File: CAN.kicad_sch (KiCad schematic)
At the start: 12 parts, among them U4 SIT65HVD230DR

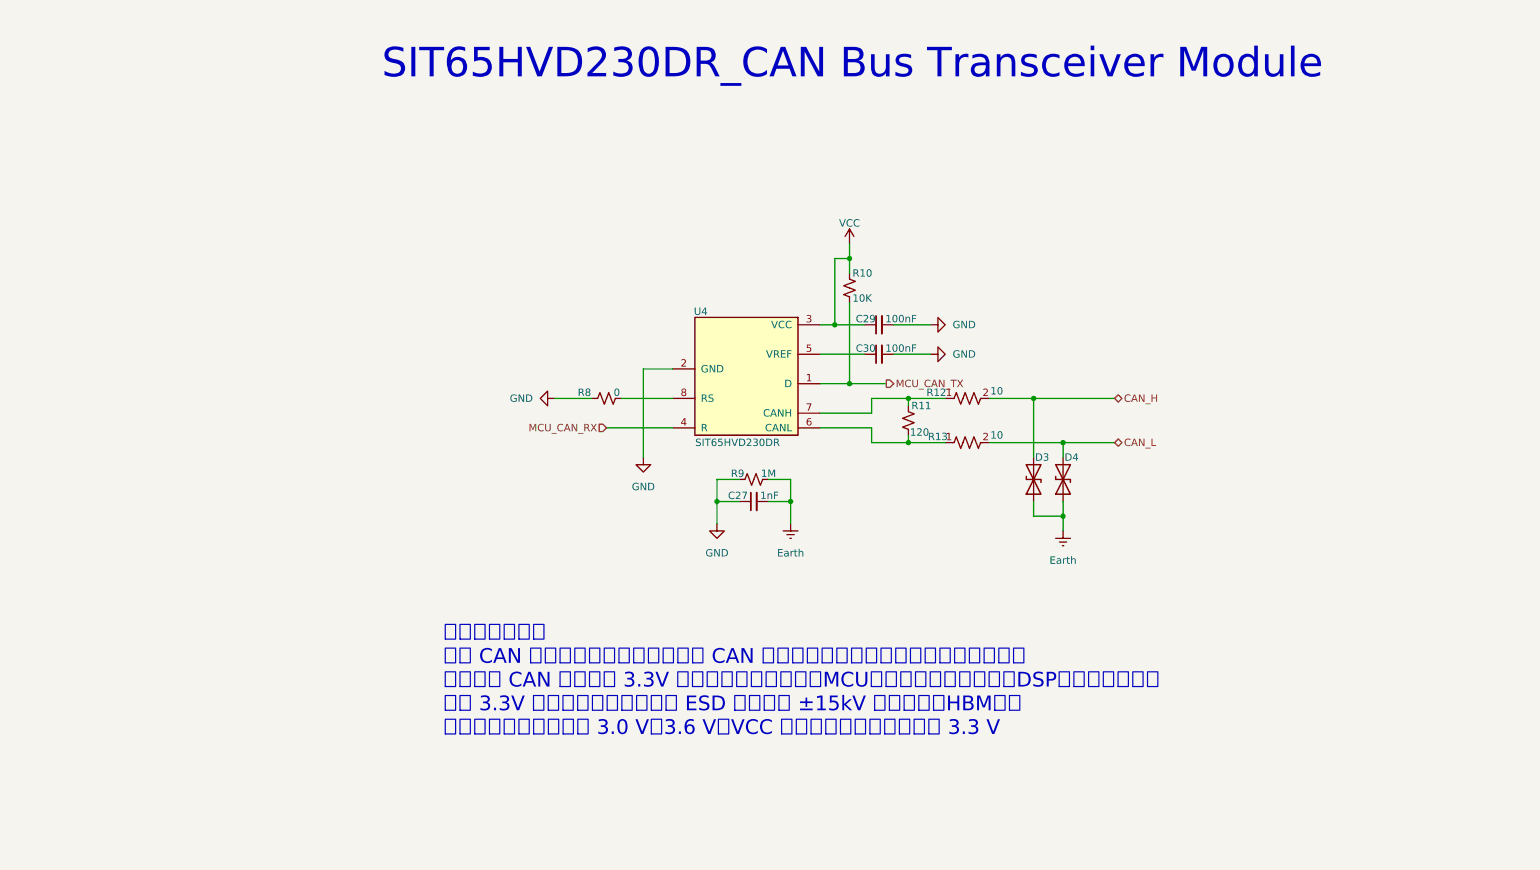
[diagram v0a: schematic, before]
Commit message: 更新原理图
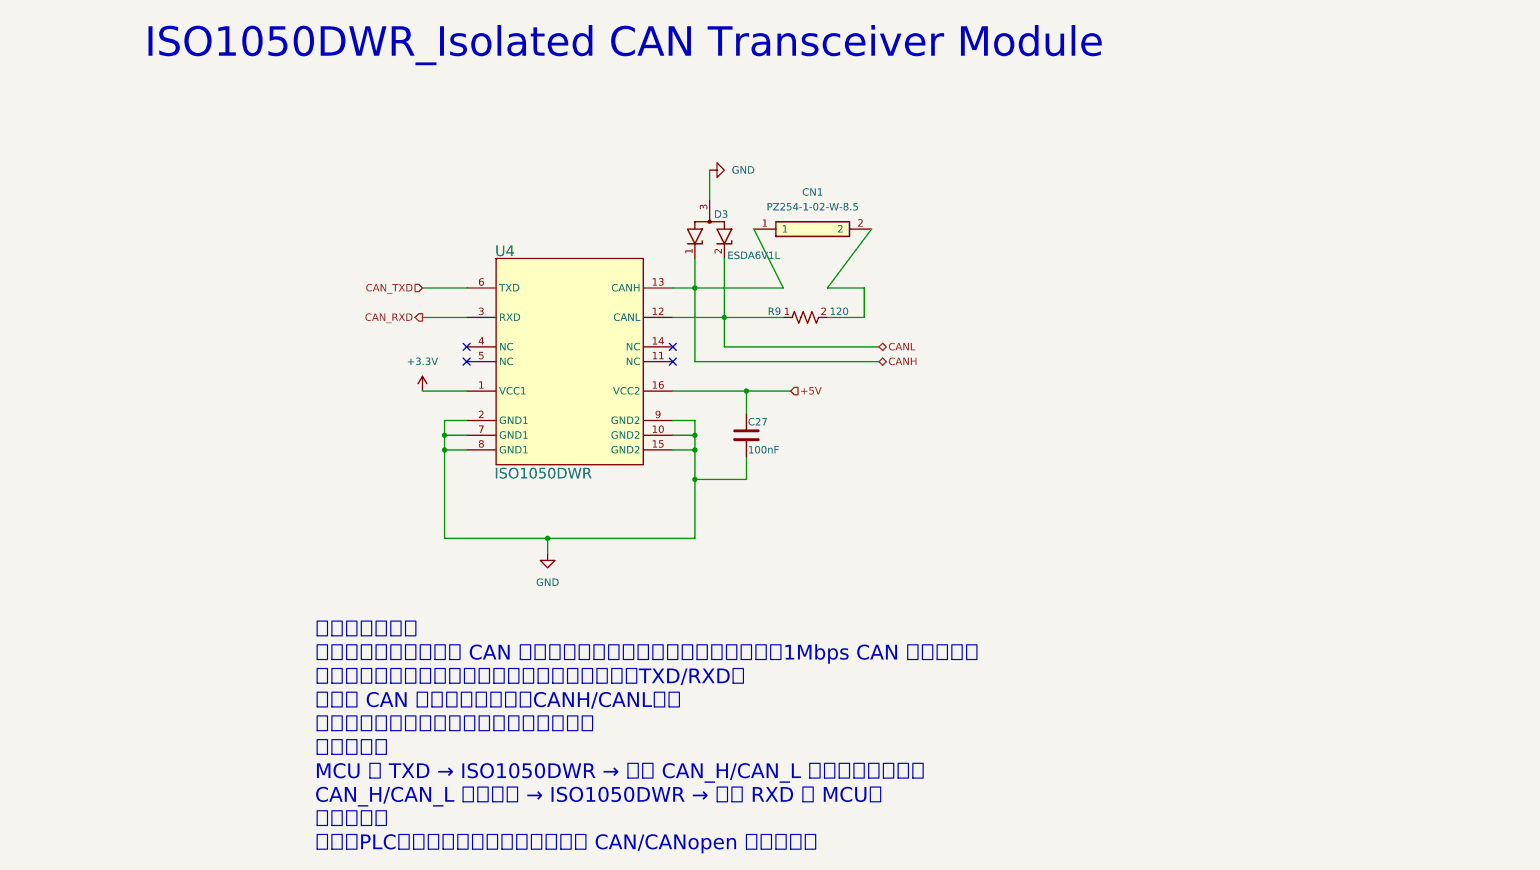
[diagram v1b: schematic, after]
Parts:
- removed C27: 1nF, kicad_community_lib:CC1206JKX7RDBB102, symbol CC1206JKX7RDBB102:CC1206JKX7RDBB102
- removed C29, C30: 100nF, kicad_api_lib:0402B104J160CT, symbol 0402B104J160CT:0402B104J160CT
- removed D3, D4: PESD12VV1BL-N, kicad_api_lib:PESD12VV1BL-N, symbol PESD12VV1BL-N:PESD12VV1BL-N
- removed R10: 10K, kicad_api_lib:AC0603JR-0710KL, symbol AC0603JR-0710KL:AC0603JR-0710KL
- removed R11: 120, kicad_api_lib:CRCW0603120RFKEA, symbol CRCW0603120RFKEA:CRCW0603120RFKEA
- removed R12, R13: 10, kicad_api_lib:AC0402FR-0710RL, symbol AC0402FR-0710RL:AC0402FR-0710RL
- removed R8: 0, kicad_api_lib:AC0603FR-070RL, symbol AC0603FR-070RL:AC0603FR-070RL
- removed R9: 1M, kicad_community_lib:RK73B1JTTD105J, symbol RK73B1JTTD105J:RK73B1JTTD105J
- removed U4: SIT65HVD230DR, kicad_api_lib:SIT65HVD230DR, symbol SIT65HVD230DR:SIT65HVD230DR
- added C27: 100nF, kicad_api_lib:CL05B104KB54PNC, symbol CL05B104KB54PNC:CL05B104KB54PNC
- added CN1: PZ254-1-02-W-8.5, kicad_api_lib:PZ254-1-02-W-8.5, symbol PZ254-1-02-W-8.5:FWF12507-S02B24W5B
- added D3: ESDA6V1L, kicad_api_lib:ESDA6V1L, symbol ESDA6V1L:ESDA6V1L
- added R9: 120, kicad_api_lib:0603WAF1200T5E, symbol 0603WAF1200T5E:0603WAF1200T5E
- added U4: ISO1050DWR, kicad_api_lib:ISO1050DWR, symbol ISO1050DWR:ISO1050DWR
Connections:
- net GND: now also C27.2, D3.3 (A), U4.10 (GND2), U4.15 (GND2), U4.2 (GND1), U4.7 (GND1), U4.8 (GND1), U4.9 (GND2)
- new net: CN1.2, R9.2
- new net +3.3V: U4.1 (VCC1)
- new net +5V: C27.1, U4.16 (VCC2)
- new net CANH: CN1.1, D3.1 (K1), U4.13 (CANH)
- new net CANL: D3.2 (K2), R9.1, U4.12 (CANL)
- new net CAN_RXD: U4.3 (RXD)
- new net CAN_TXD: U4.6 (TXD)
- no-connect marks 0 -> 4
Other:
- note added: "ISO1050DWR_Isolated CAN Transceiver Module"
- note added: "模块电路功能： 这是一个带隔离功能的 CAN 总线收发器电路，采用半双工，最高支持1Mbps CAN 通信速率； 该电路的主要功能是将微控制器的逻辑电平信号（TXD/RXD） 转换为 CAN 总线的差分信号（CANH/CANL）， 同时在逻辑侧和总线侧之间提供电气隔离。 引脚功能： MCU 的 TXD → ISO1050DWR → 驱动 CAN_H/CAN_L 差分信号上总线。 CAN_H/CAN_L 差分信号 → ISO1050DWR → 输出 RXD 给 MCU。 应用场景： 适用于PLC、伺服驱动器、工业机器人的 CAN/CANopen 通信隔离；"
- note removed: "SIT65HVD230DR_CAN Bus Transceiver Module"
- note removed: "模块电路功能： 一款 CAN 总线收发器芯片，该芯片是 CAN 协议控制器和物理总线之间的接口芯片， 可与具有 CAN 控制器的 3.3V 微处理器、微控制器（MCU）和数字信号处理器（DSP）等结合使用， 采用 3.3V 单电源供电，总线引脚 ESD 保护超过 ±15kV 人体模型（HBM）， 单电源工作电压范围为 3.0 V～3.6 V（VCC 引脚），典型工作电压为 3.3 V"
